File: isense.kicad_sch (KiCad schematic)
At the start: 21 parts, among them U1 TLV2372, U7 INA138, U8 LM2904, U9 LM393LV

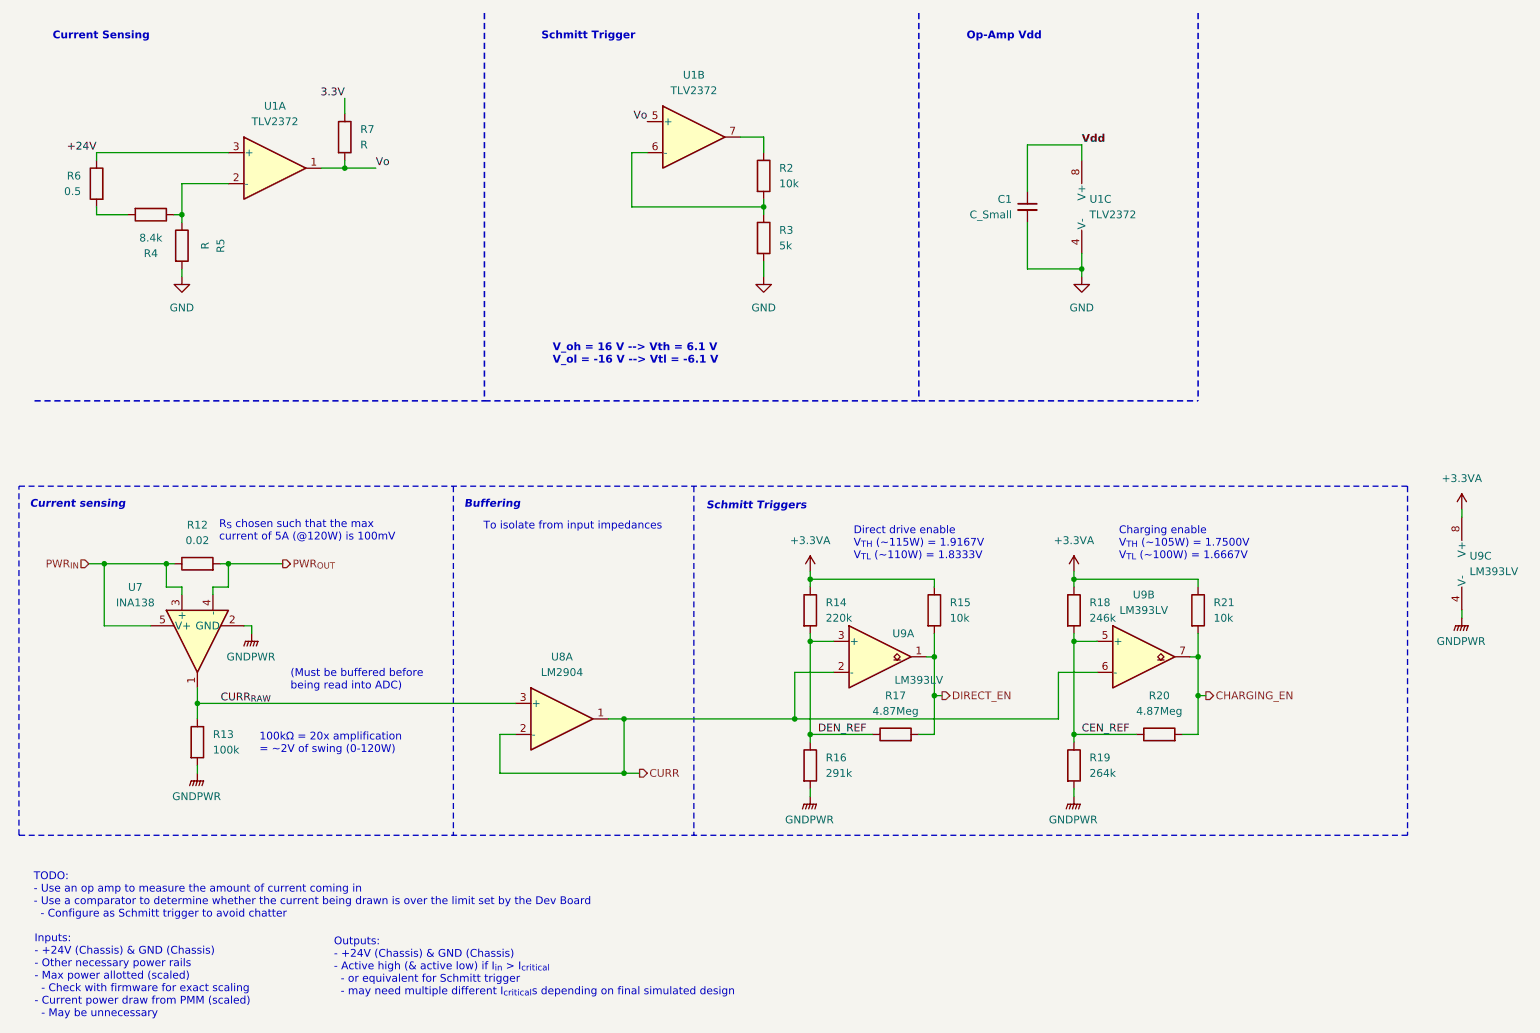
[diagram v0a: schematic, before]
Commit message: Fix ground references
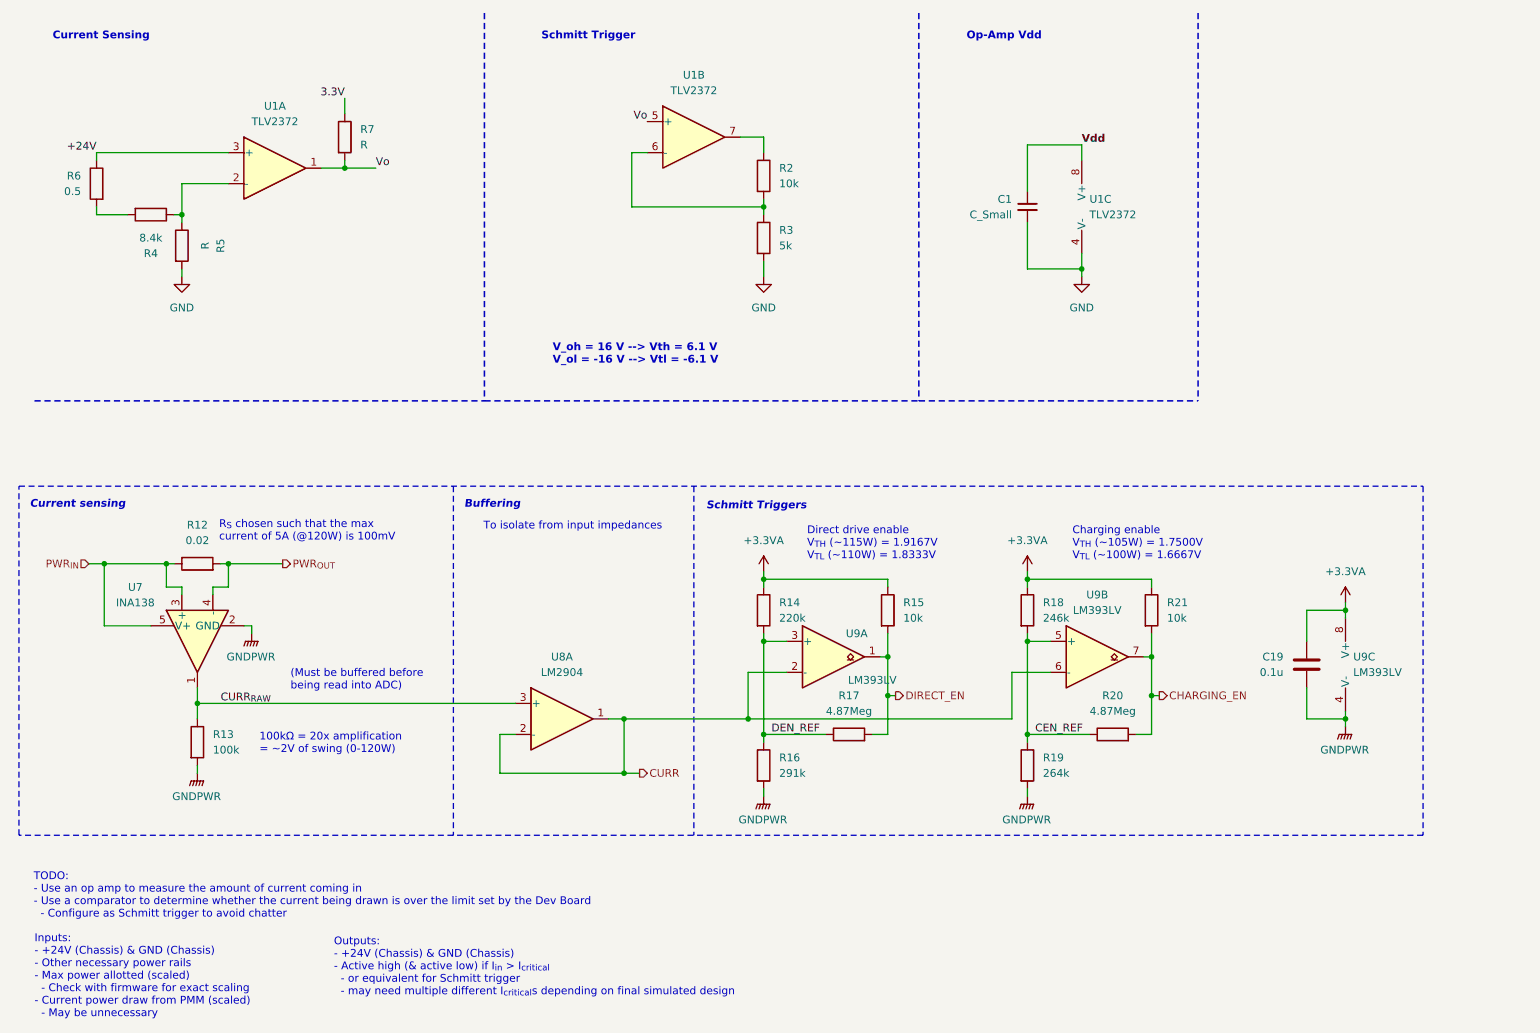
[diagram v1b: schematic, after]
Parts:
- added C19: 0.1u, symbol Device:C
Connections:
- net +3.3VA: now also C19.2
- net GNDPWR: now also C19.1
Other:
- moved on the sheet: R14, R15, R16, R17, R18, R19, R20, R21, U9A, U9B, U9C

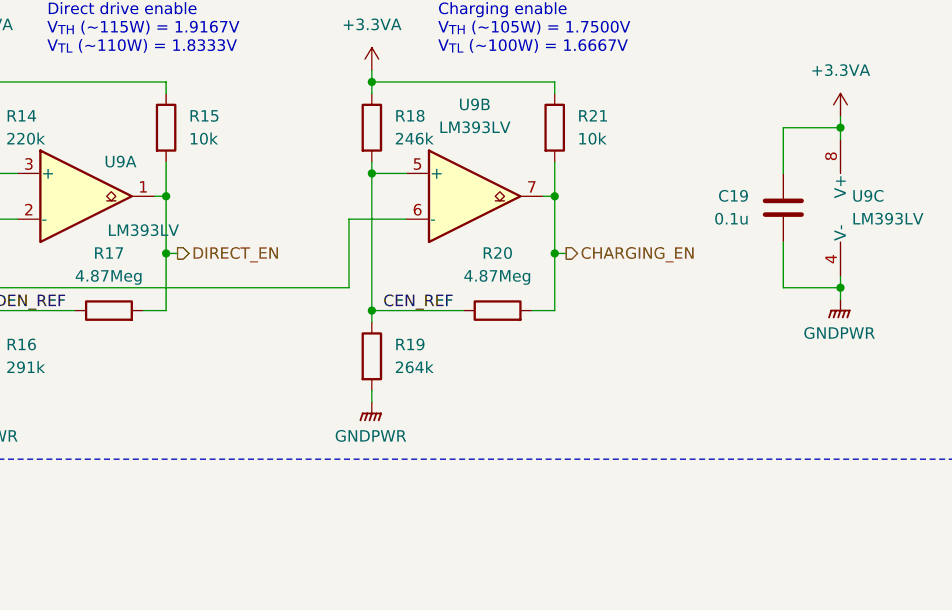
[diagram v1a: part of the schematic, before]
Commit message: formatting!?!? idk what I changed tbh
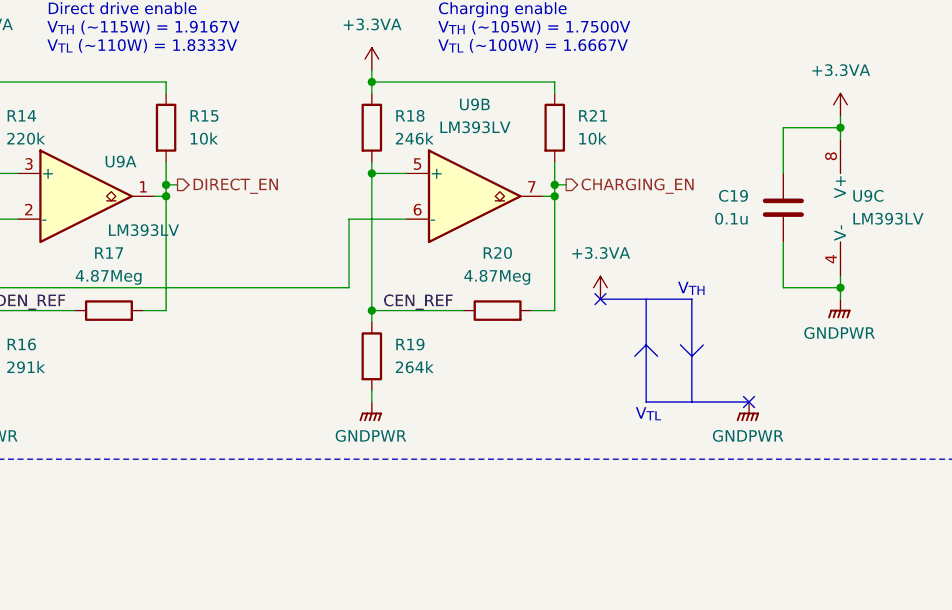
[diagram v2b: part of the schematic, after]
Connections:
- no-connect marks 0 -> 2
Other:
- note added: "V_{TH}"
- note added: "V_{TL}"
